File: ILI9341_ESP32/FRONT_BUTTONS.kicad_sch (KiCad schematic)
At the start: 23 parts, among them J5 Micro_SD_Card_CD, J6 Conn_01x18_Socket, Q2 BC817, SW10 SW_Push, SW11 SW_Push, SW12 SW_Push, SW2 SW_Push, SW3 SW_Push, SW4 SW_Push, SW5 SW_Push, SW9 SW_Push, U8 IPCB05501F20S3V, U9 IPCB05501M20S3V

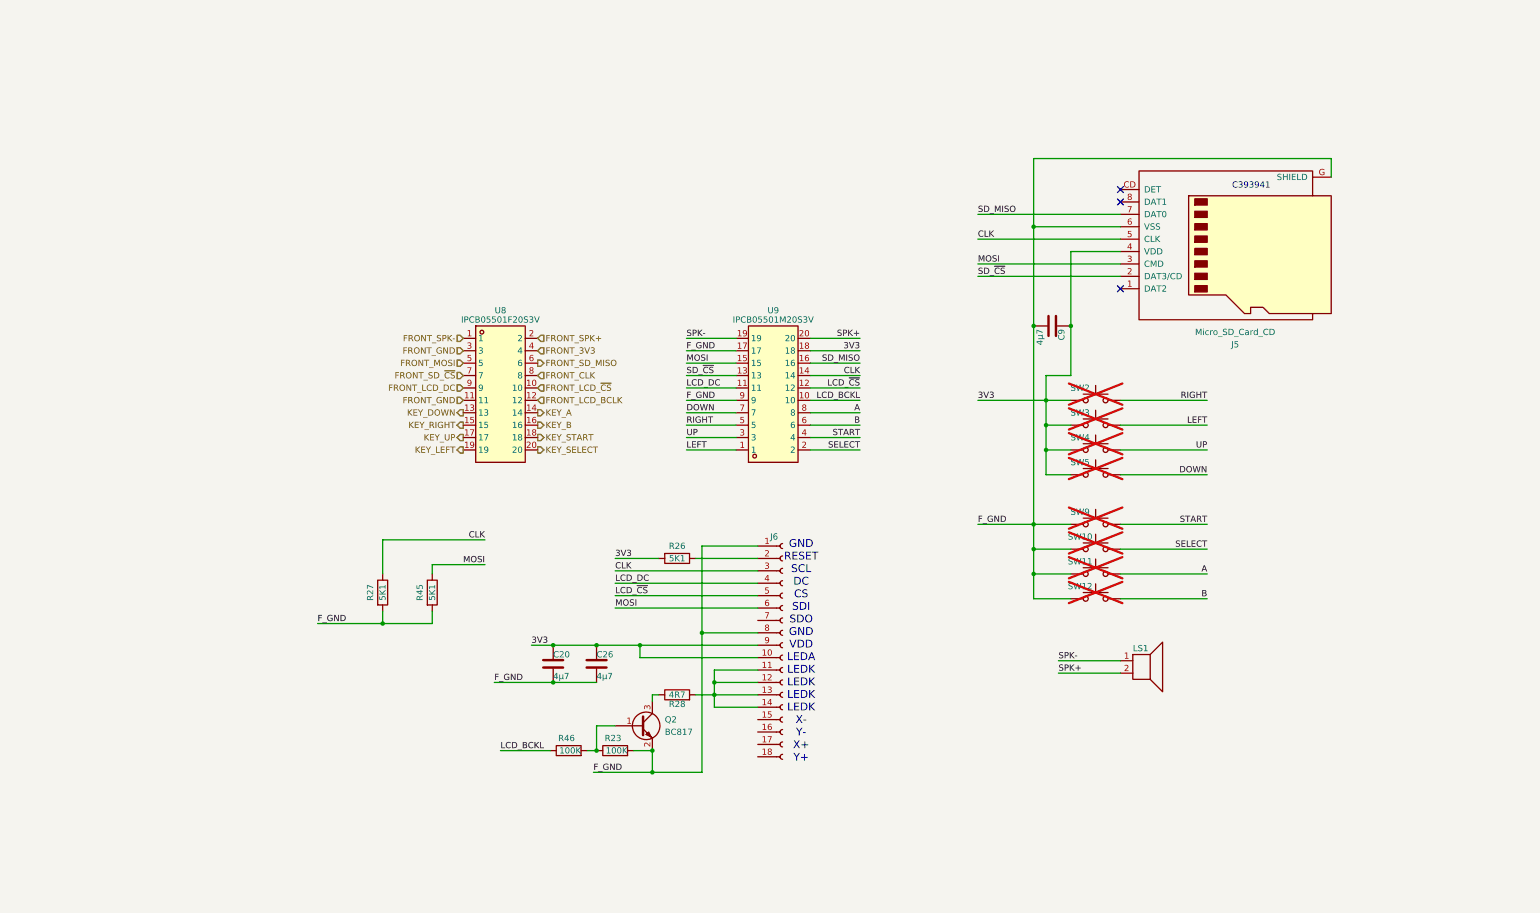
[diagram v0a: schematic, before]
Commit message: zwischenstand v2
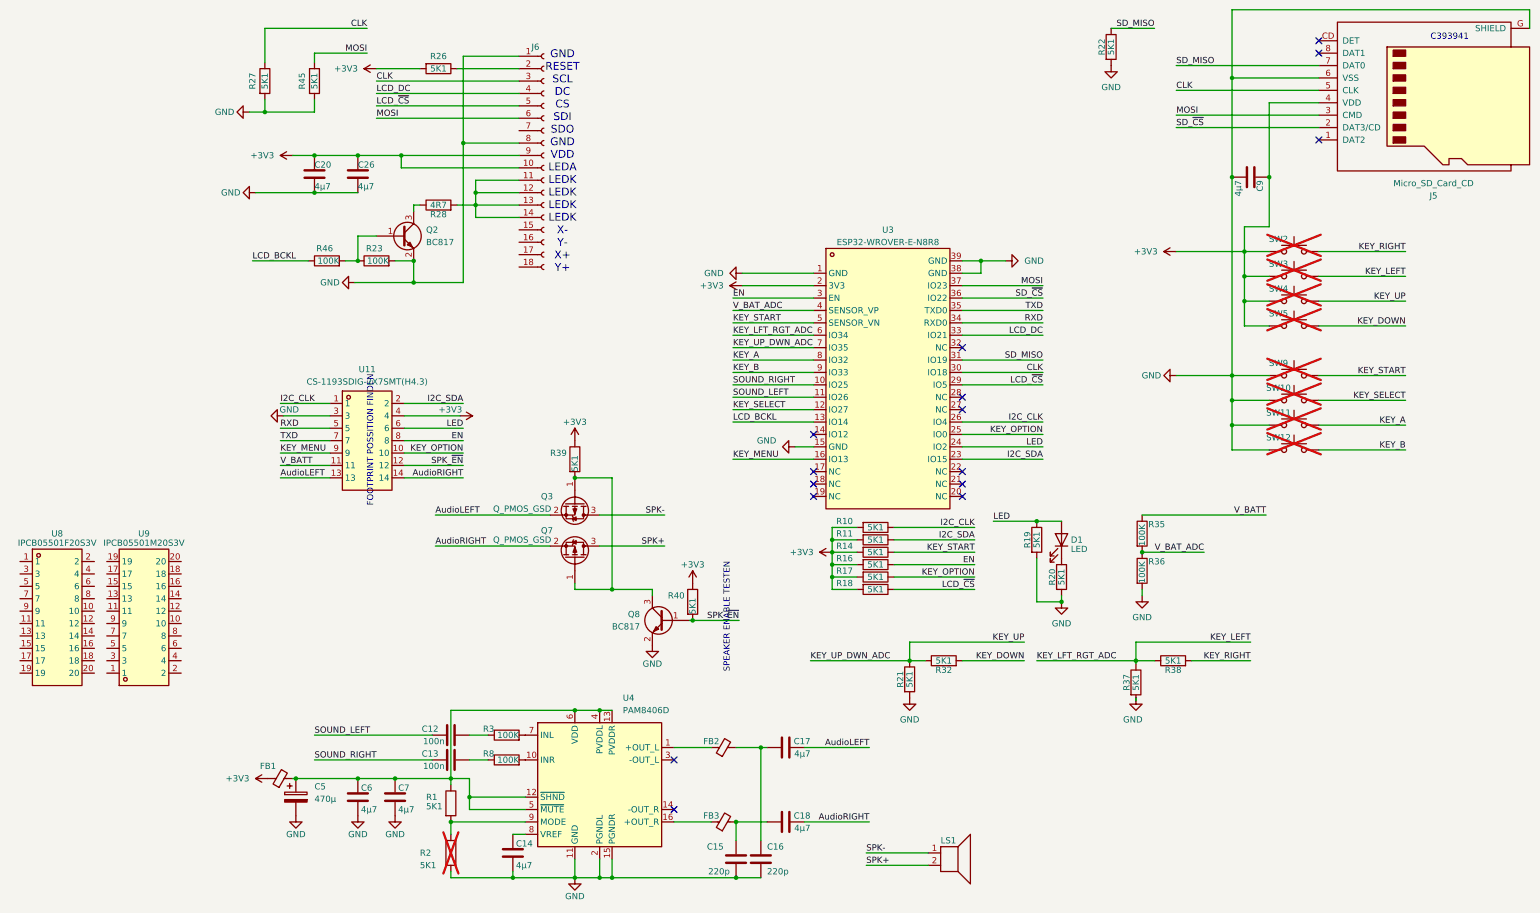
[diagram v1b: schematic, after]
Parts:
- added C12, C13: 100n, Capacitor_SMD:C_1206_3216Metric, symbol Device:C
- added C14, C17, C18, C6, C7: 4µ7, Capacitor_SMD:C_1206_3216Metric, symbol Device:C
- added C15, C16: 220p, Capacitor_SMD:C_0603_1608Metric, symbol Device:C
- added C5: 470µ, Capacitor_Tantalum_SMD:CP_EIA-7343-43_Kemet-X, symbol Device:C_Polarized
- added D1: LED, LED_SMD:LED_0603_1608Metric, symbol Device:LED
- added FB1, FB2, FB3: FerriteBead_Small, Inductor_SMD:L_0805_2012Metric, symbol Device:FerriteBead_Small
- added Q3, Q7: Q_PMOS_GSD, Package_TO_SOT_SMD:SOT-323_SC-70, symbol Device:Q_PMOS_GSD
- added Q8: BC817, Package_TO_SOT_SMD:SOT-323_SC-70, symbol Transistor_BJT:BC817
- added R1, R2, R39, R40: 5K1, Resistor_SMD:R_0603_1608Metric, symbol Device:R
- added R10, R11, R14, R16, R17, R18, R19, R20, R21, R22, R32, R37, R38: 5K1, Resistor_SMD:R_0603_1608Metric_Pad0.98x0.95mm_HandSolder, symbol Device:R
- added R3, R35, R36, R8: 100K, Resistor_SMD:R_0603_1608Metric_Pad0.98x0.95mm_HandSolder, symbol Device:R
- added U11: CS-1193SDIG-2X7SMT(H4.3), TheBrutzlers_Lib:PM200-2-07-S-4.3, symbol easyeda2kicad:CS-1193SDIG-2X7SMT(H4.3)
- added U3: ESP32-WROVER-E-N8R8, easyeda2kicad:WIFI-SMD_ESP32-WROVER-IE8MB, symbol easyeda2kicad:ESP32-WROVER-E-N8R8
- added U4: PAM8406D, Package_SO:SOP-16_3.9x9.9mm_P1.27mm, symbol Amplifier_Audio:PAM8406D
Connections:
- net CLK: now also U3.30 (IO18); no longer U9.14
- net KEY_A: now also SW11.2, U3.8 (IO32); no longer U8.14
- net KEY_B: now also SW12.2, U3.9 (IO33); no longer U8.16
- net KEY_DOWN: now also SW5.2, R32.2; no longer U8.13
- net KEY_LEFT: now also SW3.2, R37.1, R38.1, U3.6 (IO34); no longer U8.19
- net KEY_RIGHT: now also SW2.2, R38.2; no longer U8.15
- net KEY_SELECT: now also SW10.2, U3.12 (IO27); no longer U8.20
- net KEY_START: now also SW9.2, R14.1, U3.5 (SENSOR_VN); no longer U8.18
- net KEY_UP: now also SW4.2, R21.1, R32.1, U3.7 (IO35); no longer U8.17
- net LCD_BCKL: now also U3.13 (IO14); no longer U9.10
- net LCD_DC: now also U3.33 (IO21); no longer U9.11
- net LCD_~{CS}: now also R18.1, U3.29 (IO5); no longer U9.12
- net MOSI: now also U3.37 (IO23); no longer U9.15
- net SD_MISO: now also R22.1, U3.31 (IO19); no longer U9.16
- net SD_~{CS}: now also U3.36 (IO22); no longer U9.13
- net SPK+: now also Q7.3 (D); no longer U9.20
- net SPK-: now also Q3.3 (D); no longer U9.19
- net 3V3 renamed +3V3
- net +3V3: now also FB1.1, R10.2, R11.2, R14.2, R16.2, R17.2, R18.2, R39.1, R40.1, U11.4, U3.2 (3V3); no longer U9.18
- net A: no longer names the net of U9.8
- net A: no longer SW11.2
- net B: no longer names the net of U9.6
- net B: no longer SW12.2
- net DOWN: no longer names the net of U9.7
- net DOWN: no longer SW5.2
- net FRONT_3V3: no longer names the net of U8.4
- net FRONT_CLK: no longer names the net of U8.8
- net FRONT_GND: no longer names the net of U8.11
- net FRONT_GND: no longer U8.3
- net FRONT_LCD_BCLK: no longer names the net of U8.12
- net FRONT_LCD_DC: no longer names the net of U8.9
- net FRONT_LCD_~{CS}: no longer names the net of U8.10
- net FRONT_MOSI: no longer names the net of U8.5
- net FRONT_SD_MISO: no longer names the net of U8.6
- net FRONT_SD_~{CS}: no longer names the net of U8.7
- net FRONT_SPK+: no longer names the net of U8.2
- net FRONT_SPK-: no longer names the net of U8.1
- net F_GND renamed GND
- net GND: now also C14.2, C15.2, C16.1, C5.2, C6.2, C7.2, Q8.2 (E), R19.2, R2.2, R20.2, R21.2, R22.2, R36.2, R37.2, U11.3, U3.1 (GND), U3.15 (GND), U3.38 (GND), U3.39 (GND), U4.11 (GND), U4.15 (PGNDR), U4.2 (PGNDL); no longer U9.17, U9.9
- net LEFT: no longer names the net of U9.1
- net LEFT: no longer SW3.2
- net RIGHT: no longer names the net of U9.5
- net RIGHT: no longer SW2.2
- net SELECT: no longer names the net of U9.2
- net SELECT: no longer SW10.2
- net START: no longer names the net of U9.4
- net START: no longer SW9.2
- net UP: no longer names the net of U9.3
- net UP: no longer SW4.2
- new net: C5.1, C6.1, C7.1, FB1.2, R1.1, U4.12 (~{SHND}), U4.13 (PVDDR), U4.4 (PVDDL), U4.5 (~{MUTE}), U4.6 (VDD)
- new net: FB2.1, U4.1 (+OUT_L)
- new net: C16.2, C17.1, FB2.2
- new net: C15.1, C18.1, FB3.2
- new net: C12.2, R3.1
- new net: R3.2, U4.7 (INL)
- new net: Q3.1 (G), Q7.1 (G), Q8.3 (C), R39.2
- new net: D1.1 (K), R20.1
- new net: R1.2, R2.1, U4.9 (MODE)
- new net: C13.2, R8.1
- new net: R8.2, U4.10 (INR)
- new net: C14.1, U4.8 (VREF)
- new net: FB3.1, U4.16 (+OUT_R)
- new net AudioLEFT: C17.2, Q3.2 (S), U11.13
- new net AudioRIGHT: C18.2, Q7.2 (S), U11.14
- new net EN: R16.1, U11.8, U3.3 (EN)
- new net I2C_CLK: R10.1, U11.1, U3.26 (IO4)
- new net I2C_SDA: R11.1, U11.2, U3.23 (IO15)
- new net KEY_MENU: U11.9, U3.16 (IO13)
- new net KEY_OPTION: R17.1, U11.10, U3.25 (IO0)
- new net LED: D1.2 (A), R19.1, U11.6, U3.24 (IO2)
- new net RXD: U11.5, U3.34 (RXD0)
- new net SOUND_LEFT: C12.1, U3.11 (IO26)
- new net SOUND_RIGHT: C13.1, U3.10 (IO25)
- new net SPK_~{EN}: Q8.1 (B), R40.2, U11.12
- new net TXD: U11.7, U3.35 (TXD0)
- new net V_BATT: R35.1, U11.11
- new net V_BAT_ADC: R35.2, R36.1, U3.4 (SENSOR_VP)
- no-connect marks 3 -> 15
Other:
- note added: "FOOTPRINT POSSITION FINDEN"
- note added: "SPEAKER ENABLE TESTEN"
- moved on the sheet: C20, C26, C9, J5, J6, LS1, Q2, R23, R26, R27, R28, R45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
